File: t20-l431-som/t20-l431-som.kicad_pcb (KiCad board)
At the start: 4 copper layers, 10.1 x 12.2 mm, 54 parts, among them U1 STM32L431-WLCSP64, U2 T20W80, U3 MX25U3232F, U4 MODULE_INTERNAL_T20_L431_HOST, U5 LP3986TL-2518/NOPB, U6 74LVC1T45_DSBGA_YZP, U7 TPS22916BYFPR, U8 SIT8021AI-J4-XXS-16.000000, U9 NCP139AFCT120T2G

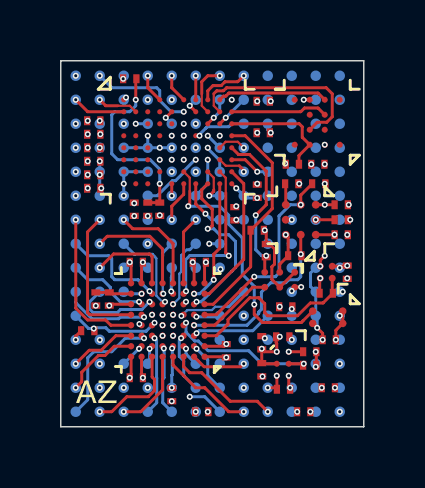
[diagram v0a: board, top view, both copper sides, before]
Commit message: Various layout fixes for DRC
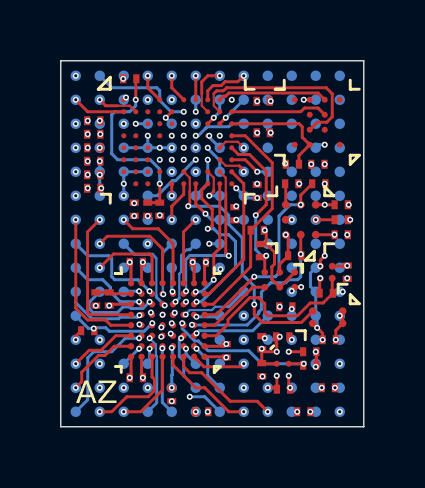
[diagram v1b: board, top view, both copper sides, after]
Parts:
- moved R7 0.20 mm to (89.2, 73.1)
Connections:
- U4 pad D11: (no net) -> /1V8
- U4 pad E10: (no net) -> /1V8
- U4 pad E11: (no net) -> /GND
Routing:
- net /1V8: track 13.0 -> 13.9 mm
- net /FPGA IO/GPIOL_21_CTRL1_CDI5: vias 2 -> 1
- net /3V3: vias 20 -> 19
